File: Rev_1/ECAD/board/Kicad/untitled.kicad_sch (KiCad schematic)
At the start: 53 parts, among them Q2 IPP029N15NM6, Q3 NPN, Q4 PNP, Q5 NMOS, U1 LM3478MA, U6 LM358

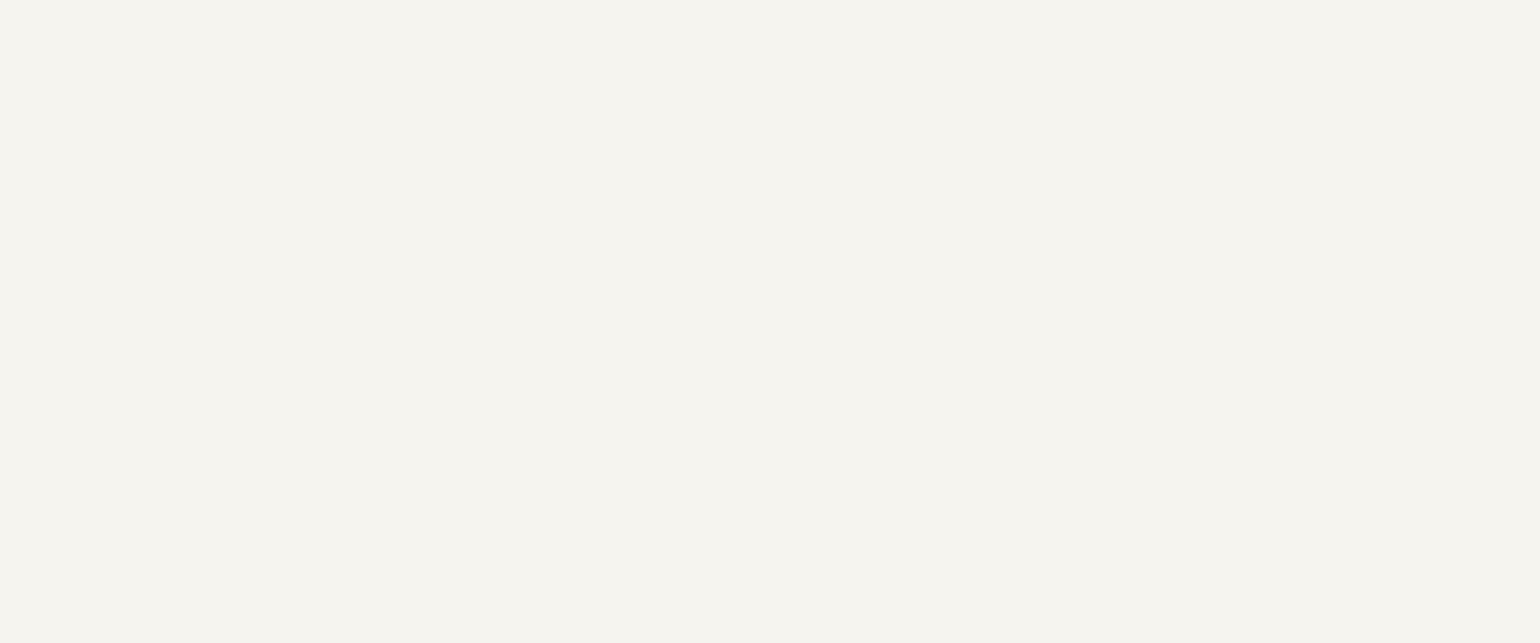
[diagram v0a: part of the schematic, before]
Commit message: made sketch of cuk converter
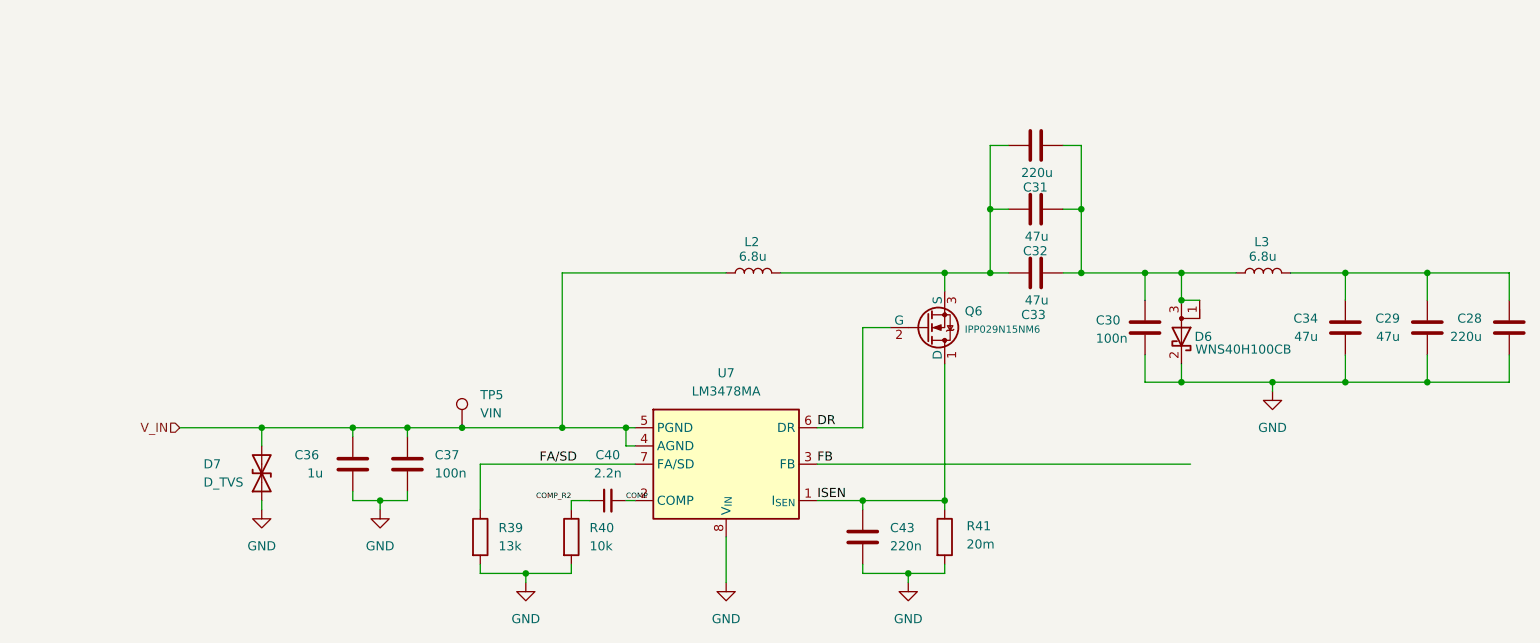
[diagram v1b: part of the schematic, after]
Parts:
- added C28, C31: 220u, Capacitor_SMD:CP_Elec_10x10.5, symbol Device:C
- added C29, C32, C33, C34: 47u, Capacitor_SMD:C_1210_3225Metric_Pad1.33x2.70mm_HandSolder, symbol Device:C
- added C30: 100n, symbol Device:C
- added C36: 1u, Capacitor_SMD:C_0603_1608Metric_Pad1.08x0.95mm_HandSolder, symbol Device:C
- added C37: 100n, Capacitor_SMD:C_0603_1608Metric_Pad1.08x0.95mm_HandSolder, symbol Device:C
- added C40: 2.2n, Capacitor_SMD:C_0603_1608Metric_Pad1.08x0.95mm_HandSolder, symbol Device:C_Small
- added C43: 220n, Capacitor_SMD:C_0603_1608Metric_Pad1.08x0.95mm_HandSolder, symbol Device:C
- added D6: WNS40H100CB, Package_TO_SOT_THT:TO-220-3_Vertical, symbol Device:D_Schottky_AKA
- added D7: D_TVS, Diode_SMD:D_0805_2012Metric_Pad1.15x1.40mm_HandSolder, symbol Device:D_TVS
- added L2, L3: 6.8u, filip:L_IHLP5050FD_5.0x5.0mm_Shielded, symbol Device:L
- added Q6: IPP029N15NM6, filip:TO-263-4_TabPin1-HandSoldered, symbol Simulation_SPICE:NMOS
- added R39: 13k, Resistor_SMD:R_0603_1608Metric_Pad0.98x0.95mm_HandSolder, symbol Device:R
- added R40: 10k, Resistor_SMD:R_0805_2012Metric_Pad1.20x1.40mm_HandSolder, symbol Device:R
- added R41: 20m, Resistor_SMD:R_1206_3216Metric_Pad1.30x1.75mm_HandSolder, symbol Device:R
- added TP5: VIN, Connector_Pin:Pin_D0.7mm_L6.5mm_W1.8mm_FlatFork, symbol Connector:TestPoint
- added U7: LM3478MA, Package_SO:SOIC-8_3.9x4.9mm_P1.27mm, symbol Regulator_Controller:LM3478MA
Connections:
- net COMP: now also C40.2, U7.2 (COMP)
- net COMP_R2: now also C40.1, R40.1
- net DR: now also Q6.2 (G), U7.6 (DR)
- net FA/SD: now also R39.1, U7.7 (FA/SD)
- net FB: now also U7.3 (FB)
- net GND: now also C28.2, C29.2, C30.2, C34.2, C36.2, C37.2, C43.2, D6.2 (K), D7.1 (A1), R39.2, R40.2, R41.2, U7.8 (V_{IN})
- net ISEN: now also C43.1, Q6.1 (D), R41.1, U7.1 (I_{SEN})
- net V_IN: now also C36.1, C37.1, D7.2 (A2), L2.2, TP5.1, U7.4 (AGND), U7.5 (PGND)
- new net: C30.1, C31.1, C32.1, C33.1, D6.1 (A), D6.3 (A), L3.2
- new net: C31.2, C32.2, C33.2, L2.1, Q6.3 (S)
- new net: C28.1, C29.1, C34.1, L3.1
